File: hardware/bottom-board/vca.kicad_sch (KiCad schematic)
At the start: 22 parts, among them Q5 2N3904, Q6 2N3906, U1 TL084, U2 NE5517

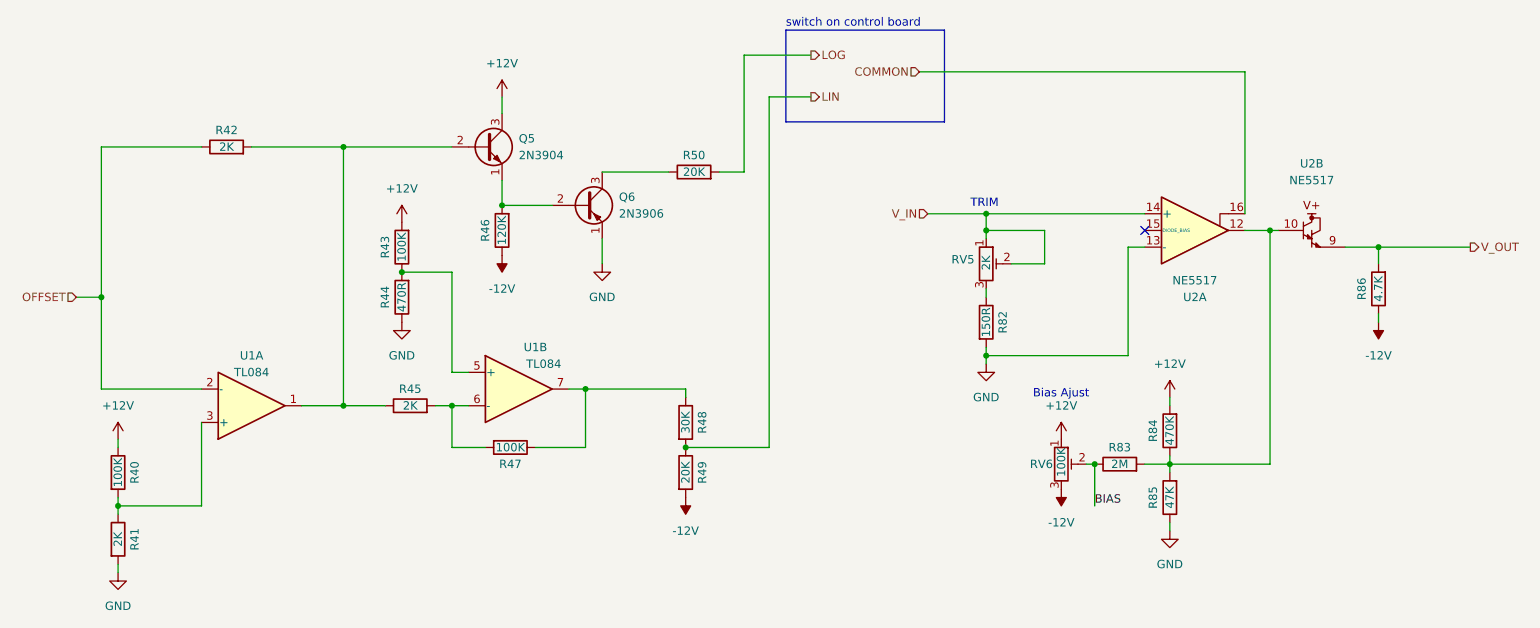
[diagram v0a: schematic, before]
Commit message: wip - first pass done
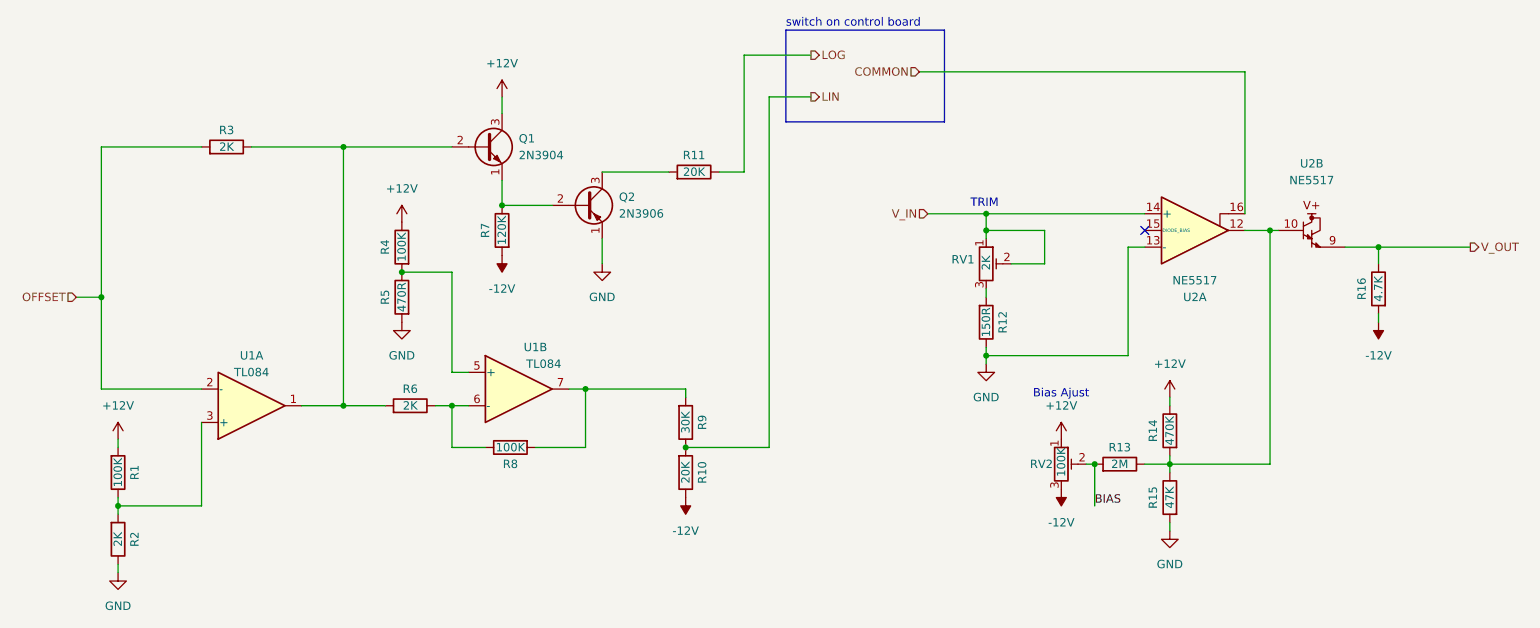
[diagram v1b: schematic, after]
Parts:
- Q1: renamed from Q5; footprint Package_TO_SOT_THT:TO-92_Inline -> Eurorack Common:TO-92_Inline; symbol Transistor_BJT:2N3904 -> Eurorack Common:2N3904
- Q2: renamed from Q6; footprint Package_TO_SOT_THT:TO-92_Inline -> Eurorack Common:TO-92_Inline; symbol Transistor_BJT:2N3906 -> Eurorack Common:2N3906
- R1: renamed from R40; footprint Resistor_THT:R_Axial_DIN0207_L6.3mm_D2.5mm_P7.62mm_Horizontal -> Eurorack Common:R_Axial_DIN0207_L6.3mm_D2.5mm_P7.62mm_Horizontal; symbol Device:R -> Eurorack Common:R_DIN0207
- R10: renamed from R49; footprint Resistor_THT:R_Axial_DIN0207_L6.3mm_D2.5mm_P7.62mm_Horizontal -> Eurorack Common:R_Axial_DIN0207_L6.3mm_D2.5mm_P7.62mm_Horizontal; symbol Device:R -> Eurorack Common:R_DIN0207
- R11: renamed from R50; footprint Resistor_THT:R_Axial_DIN0207_L6.3mm_D2.5mm_P7.62mm_Horizontal -> Eurorack Common:R_Axial_DIN0207_L6.3mm_D2.5mm_P7.62mm_Horizontal; symbol Device:R -> Eurorack Common:R_DIN0207
- R12: renamed from R82; footprint Resistor_THT:R_Axial_DIN0207_L6.3mm_D2.5mm_P7.62mm_Horizontal -> Eurorack Common:R_Axial_DIN0207_L6.3mm_D2.5mm_P7.62mm_Horizontal; symbol Device:R -> Eurorack Common:R_DIN0207
- R13: renamed from R83; footprint Resistor_THT:R_Axial_DIN0207_L6.3mm_D2.5mm_P7.62mm_Horizontal -> Eurorack Common:R_Axial_DIN0207_L6.3mm_D2.5mm_P7.62mm_Horizontal; symbol Device:R -> Eurorack Common:R_DIN0207
- R14: renamed from R84; footprint Resistor_THT:R_Axial_DIN0207_L6.3mm_D2.5mm_P7.62mm_Horizontal -> Eurorack Common:R_Axial_DIN0207_L6.3mm_D2.5mm_P7.62mm_Horizontal; symbol Device:R -> Eurorack Common:R_DIN0207
- R15: renamed from R85; footprint Resistor_THT:R_Axial_DIN0207_L6.3mm_D2.5mm_P7.62mm_Horizontal -> Eurorack Common:R_Axial_DIN0207_L6.3mm_D2.5mm_P7.62mm_Horizontal; symbol Device:R -> Eurorack Common:R_DIN0207
- R16: renamed from R86; footprint Resistor_THT:R_Axial_DIN0207_L6.3mm_D2.5mm_P7.62mm_Horizontal -> Eurorack Common:R_Axial_DIN0207_L6.3mm_D2.5mm_P7.62mm_Horizontal; symbol Device:R -> Eurorack Common:R_DIN0207
- R2: renamed from R41; footprint Resistor_THT:R_Axial_DIN0207_L6.3mm_D2.5mm_P7.62mm_Horizontal -> Eurorack Common:R_Axial_DIN0207_L6.3mm_D2.5mm_P7.62mm_Horizontal; symbol Device:R -> Eurorack Common:R_DIN0207
- R3: renamed from R42; footprint Resistor_THT:R_Axial_DIN0207_L6.3mm_D2.5mm_P7.62mm_Horizontal -> Eurorack Common:R_Axial_DIN0207_L6.3mm_D2.5mm_P7.62mm_Horizontal; symbol Device:R -> Eurorack Common:R_DIN0207
- R4: renamed from R43; footprint Resistor_THT:R_Axial_DIN0207_L6.3mm_D2.5mm_P7.62mm_Horizontal -> Eurorack Common:R_Axial_DIN0207_L6.3mm_D2.5mm_P7.62mm_Horizontal; symbol Device:R -> Eurorack Common:R_DIN0207
- R5: renamed from R44; footprint Resistor_THT:R_Axial_DIN0207_L6.3mm_D2.5mm_P7.62mm_Horizontal -> Eurorack Common:R_Axial_DIN0207_L6.3mm_D2.5mm_P7.62mm_Horizontal; symbol Device:R -> Eurorack Common:R_DIN0207
- R6: renamed from R45; footprint Resistor_THT:R_Axial_DIN0207_L6.3mm_D2.5mm_P7.62mm_Horizontal -> Eurorack Common:R_Axial_DIN0207_L6.3mm_D2.5mm_P7.62mm_Horizontal; symbol Device:R -> Eurorack Common:R_DIN0207
- R7: renamed from R46; footprint Resistor_THT:R_Axial_DIN0207_L6.3mm_D2.5mm_P7.62mm_Horizontal -> Eurorack Common:R_Axial_DIN0207_L6.3mm_D2.5mm_P7.62mm_Horizontal; symbol Device:R -> Eurorack Common:R_DIN0207
- R8: renamed from R47; footprint Resistor_THT:R_Axial_DIN0207_L6.3mm_D2.5mm_P7.62mm_Horizontal -> Eurorack Common:R_Axial_DIN0207_L6.3mm_D2.5mm_P7.62mm_Horizontal; symbol Device:R -> Eurorack Common:R_DIN0207
- R9: renamed from R48; footprint Resistor_THT:R_Axial_DIN0207_L6.3mm_D2.5mm_P7.62mm_Horizontal -> Eurorack Common:R_Axial_DIN0207_L6.3mm_D2.5mm_P7.62mm_Horizontal; symbol Device:R -> Eurorack Common:R_DIN0207
- RV1: renamed from RV5; footprint Eurorack Common:Potentiometer_Bourns_3296W_Vertical -> Eurorack Common:Potentiometer_Bourns_3296W_Horizontal
- U1: footprint Package_SO:Texas_DYY0016A_TSOT-23-16_2x4.2mm_P0.5mm -> Eurorack Common:Texas_DYY0014A_TSOT-23-14_2x4.2mm_P0.5mm; symbol Amplifier_Operational:TL084 -> Eurorack Common:TL084HIDYYR
- U2: footprint Package_SO:JEITA_SOIC-16_3.9x9.9mm_P1.27mm -> Eurorack Common:SOIC-16_3.9x9.9mm_P1.27mm; symbol Amplifier_Operational:LM13700 -> Eurorack Common:NE5517DR2G
- renumbered RV6 to RV2
